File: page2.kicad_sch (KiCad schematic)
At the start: 71 parts, among them SW1 SRBV141404, SW10 SW_SPST, SW11 SW_SPST, SW12 SW_SPST, SW13 SW_SPST, SW14 SW_SPST, SW15 SW_SPST, SW16 SW_SPST, SW17 SW_SPST, SW18 SW_SPST, SW19 SW_SPST, SW2 SW_Push_DPDT, SW3 SR2612F-0112-21R0B-D8-N, SW4 SW_SPST, SW5 SW_SPST, SW6 SW_SPST, SW7 SW_SPST, SW8 SW_SPST, SW9 SW_SPST, U1 40106, U2 4514

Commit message: routing and placing
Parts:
- D10, D11, D12, D13, D14, D15, D16, D17, D2, D3, D4, D5, D6, D7, D8, D9: footprint LED_SMD:LED_0805_2012Metric -> LED_THT:LED_D5.0mm
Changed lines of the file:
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@@
       (effects (font (size 1.27 1.27)) (justify left) hide)
     )
-    (property "Footprint" "LED_SMD:LED_0805_2012Metric" (at 140.97 109.22 0)
+    (property "Footprint" "LED_THT:LED_D5.0mm" (at 140.97 109.22 0)
       (effects (font (size 1.27 1.27)) hide)
     )
@@
       (effects (font (size 1.27 1.27)) (justify left) hide)
     )
-    (property "Footprint" "LED_SMD:LED_0805_2012Metric" (at 137.795 53.975 0)
+    (property "Footprint" "LED_THT:LED_D5.0mm" (at 137.795 53.975 0)
       (effects (font (size 1.27 1.27)) hide)
     )
@@
       (effects (font (size 1.27 1.27)) (justify left) hide)
     )
-    (property "Footprint" "LED_SMD:LED_0805_2012Metric" (at 147.32 114.3 0)
+    (property "Footprint" "LED_THT:LED_D5.0mm" (at 147.32 114.3 0)
       (effects (font (size 1.27 1.27)) hide)
     )
@@
       (effects (font (size 1.27 1.27)) (justify left) hide)
     )
-    (property "Footprint" "LED_SMD:LED_0805_2012Metric" (at 150.495 44.45 0)
+    (property "Footprint" "LED_THT:LED_D5.0mm" (at 150.495 44.45 0)
       (effects (font (size 1.27 1.27)) hide)
     )
@@
       (effects (font (size 1.27 1.27)) (justify left) hide)
     )
-    (property "Footprint" "LED_SMD:LED_0805_2012Metric" (at 153.67 119.38 0)
+    (property "Footprint" "LED_THT:LED_D5.0mm" (at 153.67 119.38 0)
       (effects (font (size 1.27 1.27)) hide)
     )
@@
       (effects (font (size 1.27 1.27)) (justify left) hide)
     )
-    (property "Footprint" "LED_SMD:LED_0805_2012Metric" (at 144.145 111.76 0)
+    (property "Footprint" "LED_THT:LED_D5.0mm" (at 144.145 111.76 0)
       (effects (font (size 1.27 1.27)) hide)
     )
@@
       (effects (font (size 1.27 1.27)) (justify left) hide)
     )
-    (property "Footprint" "LED_SMD:LED_0805_2012Metric" (at 153.67 41.91 0)
+    (property "Footprint" "LED_THT:LED_D5.0mm" (at 153.67 41.91 0)
       (effects (font (size 1.27 1.27)) hide)
     )
@@
       (effects (font (size 1.27 1.27)) (justify left) hide)
     )
-    (property "Footprint" "LED_SMD:LED_0805_2012Metric" (at 140.97 52.07 0)
+    (property "Footprint" "LED_THT:LED_D5.0mm" (at 140.97 52.07 0)
       (effects (font (size 1.27 1.27)) hide)
     )
@@
       (effects (font (size 1.27 1.27)) (justify left) hide)
     )
-    (property "Footprint" "LED_SMD:LED_0805_2012Metric" (at 134.62 56.515 0)
+    (property "Footprint" "LED_THT:LED_D5.0mm" (at 134.62 56.515 0)
       (effects (font (size 1.27 1.27)) hide)
     )
@@
       (effects (font (size 1.27 1.27)) (justify left) hide)
     )
-    (property "Footprint" "LED_SMD:LED_0805_2012Metric" (at 156.845 121.92 0)
+    (property "Footprint" "LED_THT:LED_D5.0mm" (at 156.845 121.92 0)
       (effects (font (size 1.27 1.27)) hide)
     )
@@
       (effects (font (size 1.27 1.27)) (justify left) hide)
     )
-    (property "Footprint" "LED_SMD:LED_0805_2012Metric" (at 156.845 39.37 0)
+    (property "Footprint" "LED_THT:LED_D5.0mm" (at 156.845 39.37 0)
       (effects (font (size 1.27 1.27)) hide)
     )
@@
       (effects (font (size 1.27 1.27)) (justify left) hide)
     )
-    (property "Footprint" "LED_SMD:LED_0805_2012Metric" (at 150.495 116.84 0)
+    (property "Footprint" "LED_THT:LED_D5.0mm" (at 150.495 116.84 0)
       (effects (font (size 1.27 1.27)) hide)
     )
@@
       (effects (font (size 1.27 1.27)) (justify left) hide)
     )
-    (property "Footprint" "LED_SMD:LED_0805_2012Metric" (at 137.795 107.315 0)
+    (property "Footprint" "LED_THT:LED_D5.0mm" (at 137.795 107.315 0)
       (effects (font (size 1.27 1.27)) hide)
     )
@@
       (effects (font (size 1.27 1.27)) (justify left) hide)
     )
-    (property "Footprint" "LED_SMD:LED_0805_2012Metric" (at 144.145 49.53 0)
+    (property "Footprint" "LED_THT:LED_D5.0mm" (at 144.145 49.53 0)
       (effects (font (size 1.27 1.27)) hide)
     )
@@
       (effects (font (size 1.27 1.27)) (justify left) hide)
     )
-    (property "Footprint" "LED_SMD:LED_0805_2012Metric" (at 134.62 104.775 0)
+    (property "Footprint" "LED_THT:LED_D5.0mm" (at 134.62 104.775 0)
       (effects (font (size 1.27 1.27)) hide)
     )
@@
       (effects (font (size 1.27 1.27)) (justify left) hide)
     )
-    (property "Footprint" "LED_SMD:LED_0805_2012Metric" (at 147.32 46.99 0)
+    (property "Footprint" "LED_THT:LED_D5.0mm" (at 147.32 46.99 0)
       (effects (font (size 1.27 1.27)) hide)
     )

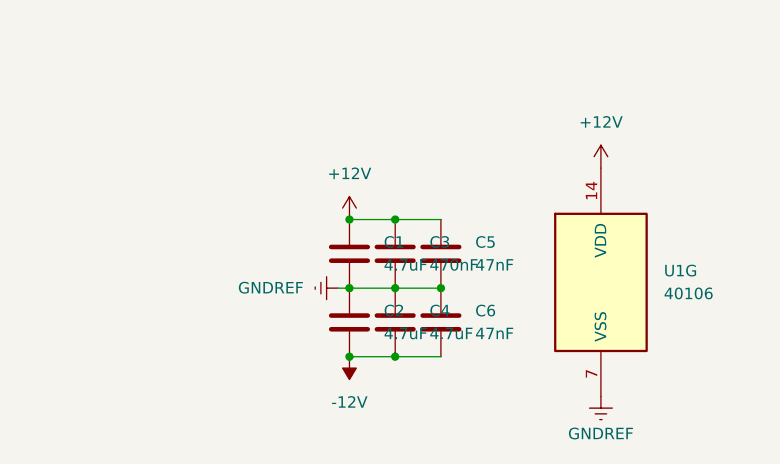
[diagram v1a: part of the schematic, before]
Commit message: routed 100%
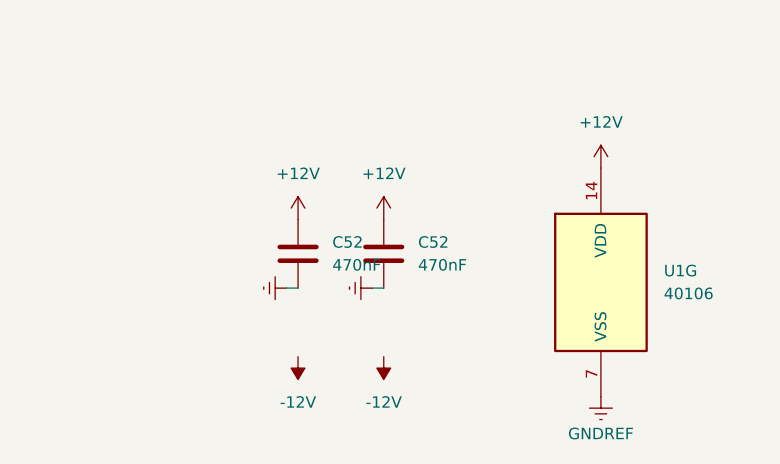
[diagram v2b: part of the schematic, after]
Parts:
- removed C1, C2, C4: 4.7uF, Capacitor_SMD:C_0805_2012Metric, symbol Device:C
- removed C3: 470nF, Capacitor_SMD:C_0805_2012Metric, symbol Device:C
- removed C5, C6: 47nF, Capacitor_SMD:C_0603_1608Metric, symbol Device:C
- added C52 (x2): 470nF, Capacitor_SMD:C_0805_2012Metric, symbol Device:C
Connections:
- net +12V: now also C52.1, C52.1
- net GNDREF: now also C52.2, C52.2
